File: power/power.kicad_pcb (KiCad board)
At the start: 2 copper layers, 165.1 x 98.5 mm, 61 parts, among them J1 ET60T-D04-3-08-D04-X-R1-S, J2 796636-6, U1 BMR4800116/005, U2 HO150-NP, U3 AZ431LANTR-G1, U3 TPS56A37RPAR, U4 RPM5.0-6.0, U5 HO8-NP, U6 AZ431LANTR-G1, U7 STM32G431KBTx, U8 AZ1117-3.3

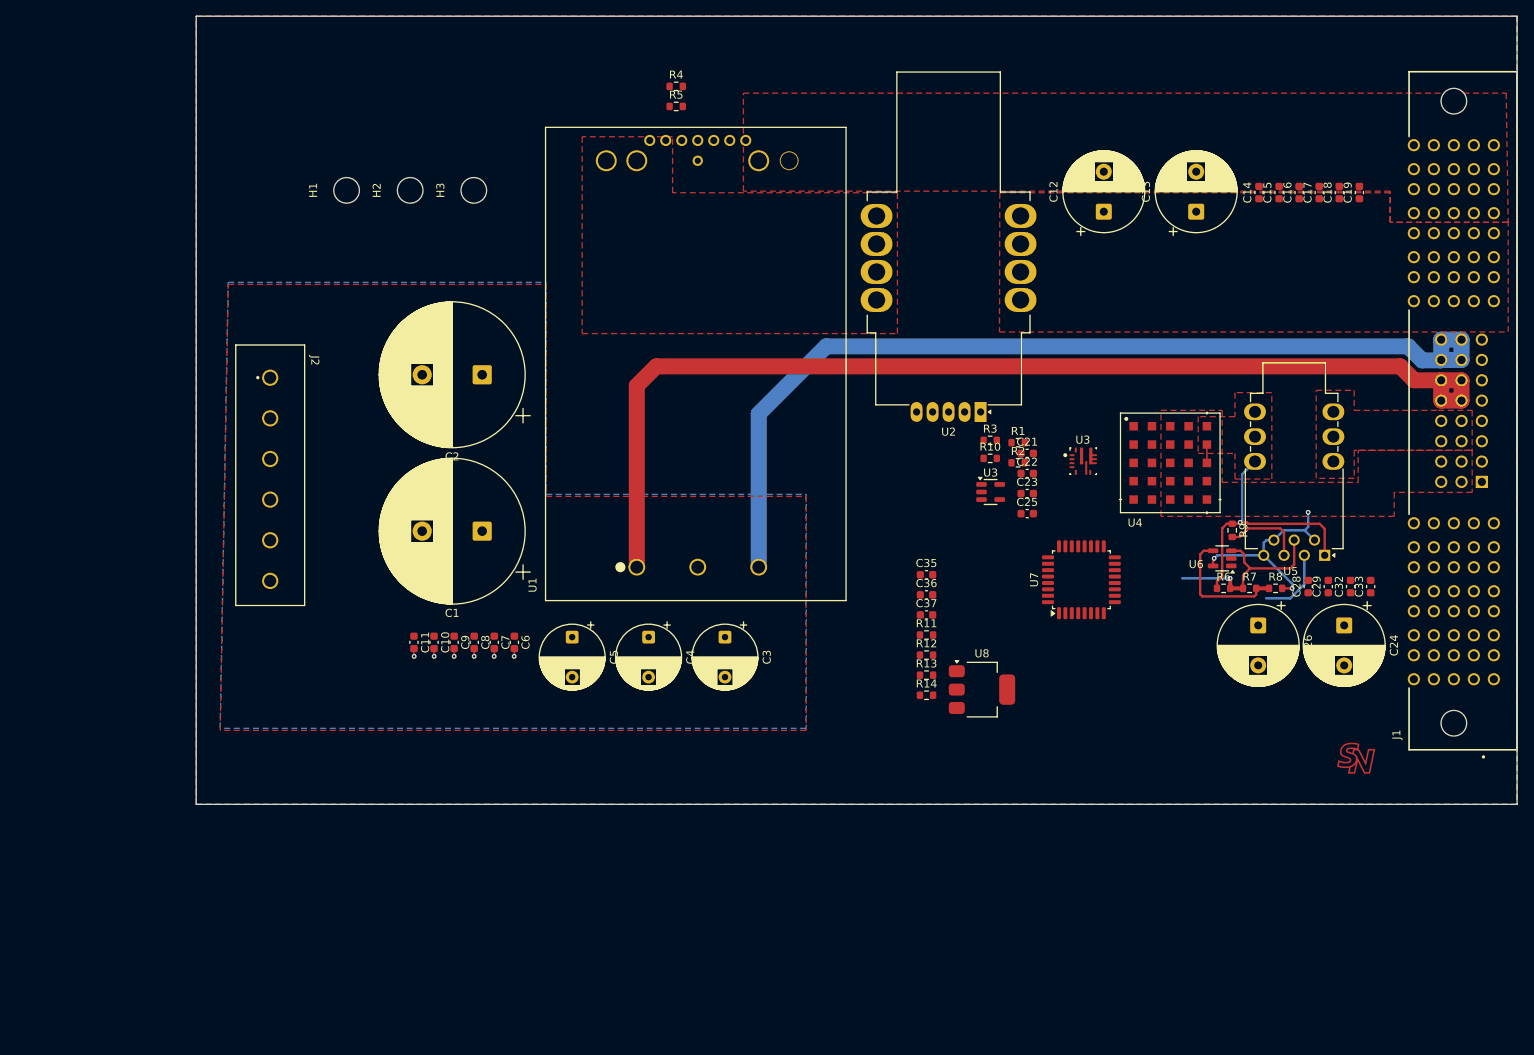
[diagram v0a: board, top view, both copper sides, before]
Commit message: update
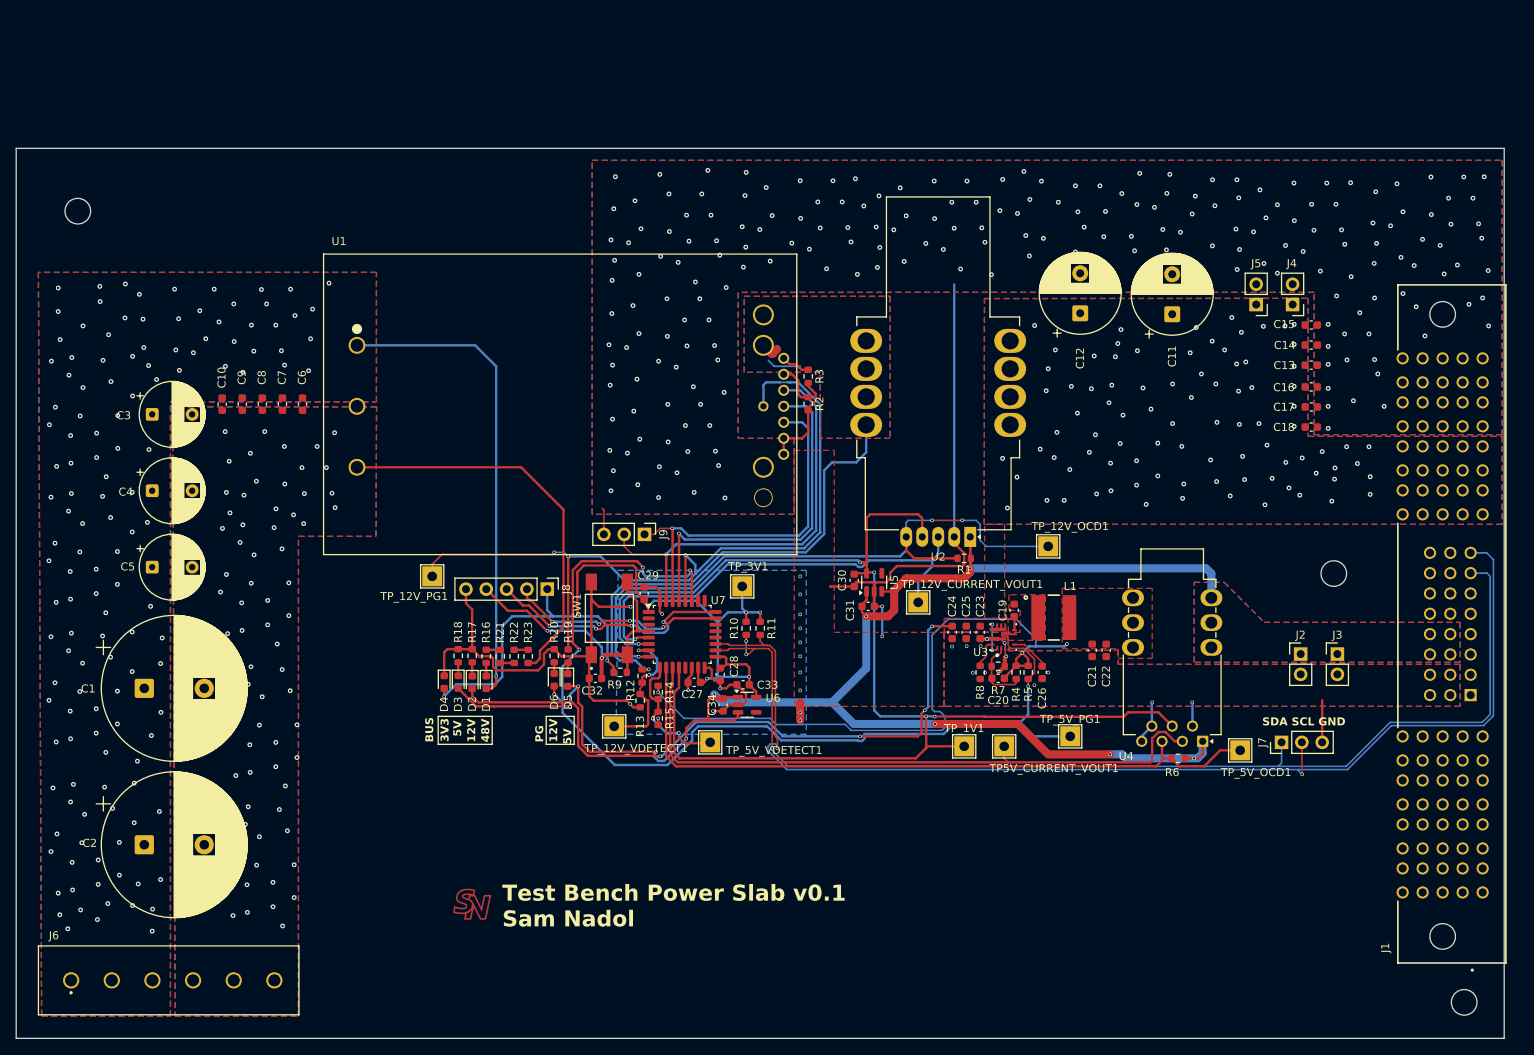
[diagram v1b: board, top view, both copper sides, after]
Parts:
- removed C35, C36, C37: C_Small, Capacitor_SMD:C_0603_1608Metric
- removed the U3 at (213.1, 75.8)
- removed the U3 at (201.6, 79.7)
- removed U8: AZ1117-3.3, Package_TO_SOT_SMD:SOT-223-3_TabPin2
- added C20: 150pF 0Ohm, Capacitor_SMD:C_0603_1608Metric, F.Cu at (202.5, 103.0)
- added C27: C_Small, Capacitor_SMD:C_0603_1608Metric, F.Cu at (164.5, 103.5)
- added C30: 10uF, Capacitor_SMD:C_0603_1608Metric, F.Cu at (184.5, 90.8)
- added C31: 10uF, Capacitor_SMD:C_0603_1608Metric, F.Cu at (186.2, 94.0)
- added C34: 10uF, Capacitor_SMD:C_0603_1608Metric, F.Cu at (168.1, 106.3)
- added D1: 48V (BLUE), LED_SMD:LED_0603_1608Metric, F.Cu at (138.5, 103.5)
- added D2: 12V (RED), LED_SMD:LED_0603_1608Metric, F.Cu at (136.8, 103.5)
- added D3: 5V (GREEN), LED_SMD:LED_0603_1608Metric, F.Cu at (135.0, 103.5)
- added D4: 3V3 (PURPLE), LED_SMD:LED_0603_1608Metric, F.Cu at (133.2, 103.5)
- added D5: 12V_PG (RED), LED_SMD:LED_0603_1608Metric, F.Cu at (148.7, 103.2)
- added D6: 5V_PG (GREEN), LED_SMD:LED_0603_1608Metric, F.Cu at (147.0, 103.2)
- added J3: misc. power output, Connector_PinHeader_2.54mm:PinHeader_1x02_P2.54mm_Vertical, F.Cu at (244.9, 100.0)
- added J4: misc. power output, Connector_PinHeader_2.54mm:PinHeader_1x02_P2.54mm_Vertical, F.Cu at (239.3, 56.3)
- added J5: misc. power output, Connector_PinHeader_2.54mm:PinHeader_1x02_P2.54mm_Vertical, F.Cu at (234.8, 56.3)
- added J6: 796636-6, power_symbols:796636-6, F.Cu at (86.6, 140.8)
- added J7: I2C, Connector_PinHeader_2.54mm:PinHeader_1x03_P2.54mm_Vertical, F.Cu at (237.9, 111.0)
- added J8: SWD, Connector_PinHeader_2.54mm:PinHeader_1x05_P2.54mm_Vertical, F.Cu at (146.1, 91.8)
- added J9: BMR_I2C, Connector_PinHeader_2.54mm:PinHeader_1x03_P2.54mm_Vertical, F.Cu at (158.3, 85.0)
- added L1: 3u3 8.6mOhm, power_symbols:WE-MXGI_5030, F.Cu at (209.4, 95.4)
- added R15: 15k, Resistor_SMD:R_0603_1608Metric, F.Cu at (160.0, 108.0)
- added R16: 680R 1/4W 0603, Resistor_SMD:R_0603_1608Metric, F.Cu at (138.5, 100.2)
- added R17: 500R, Resistor_SMD:R_0603_1608Metric, F.Cu at (136.8, 100.2)
- added R18: 120R, Resistor_SMD:R_0603_1608Metric, F.Cu at (135.0, 100.2)
- added R19: 120R, Resistor_SMD:R_0603_1608Metric, F.Cu at (148.8, 100.2)
- added R20: 120R, Resistor_SMD:R_0603_1608Metric, F.Cu at (147.0, 100.2)
- added R21: 680R 1/4W 0603, Resistor_SMD:R_0603_1608Metric, F.Cu at (140.2, 100.2)
- added R22: 680R 1/4W 0603, Resistor_SMD:R_0603_1608Metric, F.Cu at (142.0, 100.2)
- added R23: 680R 1/4W 0603, Resistor_SMD:R_0603_1608Metric, F.Cu at (143.8, 100.2)
- added SW1: SW_Push, power_symbols:TS04-66-70-BK-160-SMT, F.Cu at (153.9, 95.5)
- added TP5V_CURRENT_VOUT1: TestPoint, TestPoint:TestPoint_THTPad_2.5x2.5mm_Drill1.2mm, F.Cu at (203.2, 111.5)
- added TP_12V_CURRENT_VOUT1: TestPoint, TestPoint:TestPoint_THTPad_2.5x2.5mm_Drill1.2mm, F.Cu at (192.5, 93.5)
- added TP_12V_OCD1: TestPoint, TestPoint:TestPoint_THTPad_2.5x2.5mm_Drill1.2mm, F.Cu at (208.8, 86.5)
- added TP_12V_PG1: TestPoint, TestPoint:TestPoint_THTPad_2.5x2.5mm_Drill1.2mm, F.Cu at (131.8, 90.2)
- added TP_12V_VDETECT1: TestPoint, TestPoint:TestPoint_THTPad_2.5x2.5mm_Drill1.2mm, F.Cu at (154.5, 109.0)
- added TP_1V1: TestPoint, TestPoint:TestPoint_THTPad_2.5x2.5mm_Drill1.2mm, F.Cu at (198.2, 111.5)
- added TP_3V1: TestPoint, TestPoint:TestPoint_THTPad_2.5x2.5mm_Drill1.2mm, F.Cu at (170.5, 91.5)
- added TP_5V_OCD1: TestPoint, TestPoint:TestPoint_THTPad_2.5x2.5mm_Drill1.2mm, F.Cu at (232.8, 112.0)
- added TP_5V_PG1: TestPoint, TestPoint:TestPoint_THTPad_2.5x2.5mm_Drill1.2mm, F.Cu at (211.5, 110.2)
- added TP_5V_VDETECT1: TestPoint, TestPoint:TestPoint_THTPad_2.5x2.5mm_Drill1.2mm, F.Cu at (166.5, 111.0)
- added U3: TPS56A37RPAR, power_symbols:TPS56A37RPAR, F.Cu at (203.1, 97.8)
- C11: value C_Small -> C_Polarized_Small; footprint Capacitor_SMD:C_0603_1608Metric -> Capacitor_THT:CP_Radial_D10.0mm_P5.00mm
- C13: value C_Polarized_Small -> C_Small; footprint Capacitor_THT:CP_Radial_D10.0mm_P5.00mm -> Capacitor_SMD:C_0603_1608Metric
- C19: value C_Small -> 100nF 1mOhm
- C21, C22: value 10uF -> 22uF 2.582mOhm
- C23: value 100nF -> 10uF 2.818mOhm
- C24: value C_Polarized_Small -> 10uF 2.818mOhm; footprint Capacitor_THT:CP_Radial_D10.0mm_P5.00mm -> Capacitor_SMD:C_0603_1608Metric
- C25: value 100nF -> 1uF 5mOhm
- C26: value C_Polarized_Small -> 22nF 1mOhm; footprint Capacitor_THT:CP_Radial_D10.0mm_P5.00mm -> Capacitor_SMD:C_0603_1608Metric
- C32: value C_Small -> 3u3
- C33: value C_Small -> 10uF
- J2: value 796636-6 -> misc. power output; footprint power_symbols:796636-6 -> Connector_PinHeader_2.54mm:PinHeader_1x02_P2.54mm_Vertical
- R1, R10, R6, R9: value 22k -> 10k
- R11: value 30k -> 10k
- R12: value 10k -> 30k
- R14: value 15k -> 10k
- R2, R7: value 4k7 -> 10k
- R3: value 100k -> 10k
- R4: value 10k -> 73k2
- R5: value 10k -> 100k
- R8: value 100k -> 52k3
- U1: value BMR4800116/005 -> MPQ1500-12V125-L48NBMC
- U2: footprint custom:LEM_HO150-NP -> power_symbols:LEM_HO150-NP
- U4: value RPM5.0-6.0 -> HO15-NP; footprint power_symbols:RPM5.0-6.0 -> Sensor_Current:LEM_HO8-NP
- U5: value HO8-NP -> TPS7A24125DBVR; footprint Sensor_Current:LEM_HO8-NP -> Package_TO_SOT_SMD:SOT-23-5
- U6: value AZ431LANTR-G1 -> TPS7A2433DBVR
- moved H2 166.3 mm to (260.8, 143.5)
- moved J2 133.4 mm to (240.3, 100.0), turned to 0 degrees
- moved H3 117.7 mm to (244.4, 89.9)
- moved G1 112.0 mm to (136.8, 131.2)
- moved C11 103.3 mm to (224.2, 57.5), turned to 90 degrees
- moved C32 95.1 mm to (152.2, 103.0), turned to 180 degrees
- moved C29 85.5 mm to (158.2, 92.4)
- moved R4 84.7 mm to (204.8, 102.2), turned to -90 degrees
- moved R5 83.3 mm to (206.2, 102.2), turned to -90 degrees
- moved C33 79.4 mm to (170.6, 103.8), turned to 180 degrees
- moved R9 78.5 mm to (155.2, 102.2), turned to 0 degrees
- moved C3 76.8 mm to (96.8, 70.0), turned to 0 degrees
- moved C28 74.3 mm to (167.8, 102.5), turned to -90 degrees
- moved C2 72.4 mm to (95.8, 123.8), turned to 0 degrees
- moved C19 67.7 mm to (204.5, 94.5)
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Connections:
- C11 pad 1: +48V -> +12V
- C11 pad 2: 48V_GND -> 12V_GND
- C19 pad 1: +12V -> Net-(U3-BOOT)
- C19 pad 2: 12V_GND -> Net-(U3-SW)
- C21 pad 1: +5V -> /12-5/5V_PRESENSE
- C22 pad 1: +3V3 -> /12-5/5V_PRESENSE
- C23 pad 1: +5V -> +12V
- C24 pad 1: +5V -> +12V
- C25 pad 1: +3V3 -> +12V
- C26 pad 1: +5V -> Net-(U3-SS)
- C28 pad 1: +5V -> +3V3
- C29 pad 1: +5V -> +3V3
- C32 pad 1: +5V -> /STM/SYS_NRST
- C33 pad 1: +5V -> +3V3
- J1 pad 13: +48V -> unconnected-(J1-Pad13)
- J1 pad 14: +48V -> unconnected-(J1-Pad14)
- J1 pad 15: 48V_GND -> unconnected-(J1-Pad15)
- J1 pad 16: 48V_GND -> unconnected-(J1-Pad16)
- J1 pad 21: +48V -> unconnected-(J1-Pad21)
- J1 pad 22: +48V -> unconnected-(J1-Pad22)
- J1 pad 23: 48V_GND -> unconnected-(J1-Pad23)
- J1 pad 24: 48V_GND -> unconnected-(J1-Pad24)
- J2 pad 1: +48V -> +5V
- J2 pad 2: +48V -> 12V_GND
- R1 pad 1: /48-12/12V_CURRENT_VREF -> +5V
- R1 pad 2: +5V -> /48-12/12V_CURRENT_OCD
- R10 pad 1: /48-12/5V_PRESENSE -> +3V3
- R10 pad 2: /48-12/12V_CURRENT_OCD -> /STM_SDA
- R11 pad 1: /48-12/12V_PRESENSE -> +3V3
- R11 pad 2: /STM/12V_VDETECT -> /STM_SCL
- R12 pad 1: /STM/12V_VDETECT -> /48-12/12V_PRESENSE
- R12 pad 2: 12V_GND -> /STM/12V_VDETECT
- R13 pad 1: /12-5/5V_PRESENSE -> /STM/12V_VDETECT
- R13 pad 2: /STM/5V_VDETECT -> 12V_GND
- R14 pad 1: /STM/5V_VDETECT -> /12-5/5V_PRESENSE
- R14 pad 2: 12V_GND -> /STM/5V_VDETECT
- R2 pad 1: /48-12/12V_CURRENT_VREF -> Net-(U1-SA1)
- R2 pad 2: Net-(U3-REF) -> 12V_GND
- R3 pad 1: Net-(U3-REF) -> Net-(U1-SA0)
- R4 pad 1: Net-(U1-SA1) -> /12-5/5V_PRESENSE
- R4 pad 2: 12V_GND -> Net-(U3-FB)
- R5 pad 1: Net-(U1-SA0) -> /12-5/5V_PRESENSE
- R5 pad 2: 12V_GND -> 5V_PG
- R6 pad 1: /12-5/5V_PRESENSE -> +5V
- R6 pad 2: /12-5/5V_CURRENT_VREF -> /12-5/5V_CURRENT_OCD
- R7 pad 1: /12-5/5V_CURRENT_VREF -> Net-(U3-FB)
- R7 pad 2: Net-(U6-REF) -> 12V_GND
- R8 pad 1: Net-(U6-REF) -> Net-(U3-MODE)
- R9 pad 1: /12-5/5V_PRESENSE -> +3V3
- R9 pad 2: /12-5/5V_CURRENT_OCD -> /STM/SYS_NRST
- U1 pad 11: /48-12/BMR_SDA -> BMR_SDA
- U1 pad 12: /48-12/~{BMR_SALERT} -> ~{BMR_SALERT}
- U1 pad 13: /48-12/BMR_SCL -> BMR_SCL
- U1 pad 6: /48-12/~{BMR_PG} -> ~{BMR_PG}
- U2 pad 4: /48-12/12V_CURRENT_VREF -> +1V25
- U5 pad 1: /12-5/5V_PRESENSE -> +5V
- U5 pad 3: /12-5/5V_CURRENT_VOUT -> +5V
- U5 pad 4: /12-5/5V_CURRENT_VREF -> unconnected-(U5-FB-Pad4)
- U5 pad 5: /12-5/5V_CURRENT_OCD -> +1V25
- U6 pad 1: (no net) -> +5V
- U6 pad 2: (no net) -> 12V_GND
- U6 pad 3: /12-5/5V_CURRENT_VREF -> +5V
- U6 pad 4: Net-(U6-REF) -> unconnected-(U6-FB-Pad4)
- U6 pad 5: 12V_GND -> +3V3
- U7 pad 12: /12-5/5V_CURRENT_VREF -> +1V25
- U7 pad 27: /STM/RPM_PG -> 5V_PG
- U7 pad 28: /STM/~{BMR_PG} -> ~{BMR_PG}
- U7 pad 29: /STM/~{BMR_SALERT} -> ~{BMR_SALERT}
- U7 pad 30: /STM/BMR_SDA -> BMR_SDA
- U7 pad 31: /STM/BMR_SCL -> BMR_SCL
- U7 pad 6: /48-12/12V_CURRENT_VREF -> +1V25
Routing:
- net +5V: track 0.00 -> 206.0 mm, vias 0 -> 10
- net +1V25: track 0.00 -> 169.1 mm, vias 0 -> 5
- net 12V_GND: track 25.7 -> 184.5 mm, vias 3 -> 243
- net /STM_SCL: track 0.00 -> 145.9 mm, vias 0 -> 2
- net /STM_SDA: track 0.00 -> 139.6 mm, vias 0 -> 3
- net 5V_PG: track 0.00 -> 126.4 mm, vias 0 -> 5
- net +3V3: track 0.00 -> 106.2 mm, vias 0 -> 8
- net ~{BMR_PG}: track 0.00 -> 101.8 mm, vias 0 -> 3
- net +12V: track 0.00 -> 86.0 mm, vias 0 -> 94
- net /48-12/12V_CURRENT_OCD: track 0.00 -> 82.7 mm, vias 0 -> 3
- net /12-5/5V_CURRENT_OCD: track 10.0 -> 87.3 mm
- net +48V: track 135.1 -> 59.7 mm, vias 0 -> 135
- net 48V_GND: track 124.8 -> 49.5 mm, vias 6 -> 71
- net /12-5/5V_CURRENT_VOUT: track 9.11 -> 81.3 mm
- net /48-12/12V_PRESENSE: track 0.00 -> 70.0 mm, vias 0 -> 1
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- added copper zone on B.Cu, net +12V
- added copper zone on B.Cu, net +48V
- added copper zone on B.Cu, net +5V
- added copper zone on B.Cu, net /48-12/12V_PRESENSE
- added copper zone on F.Cu, net 48V_GND
- added copper zone on F.Cu, net Net-(U3-SW)
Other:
- board size 165.1 x 98.5 mm -> 186 x 111.2 mm
- board text added: "12V"
- board text added: "3V3"
- board text added: "48V"
- board text added: "5V"
- board text added: "BUS"
- board text added: "PG"
- board text added: "SDA SCL GND"
- board text added: "Test Bench Power Slab v0.1 Sam Nadol"
